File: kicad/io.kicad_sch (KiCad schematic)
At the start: 9 parts, among them SW1 UP, SW2 DOWN, SW3 OK, SW4 CANCEL

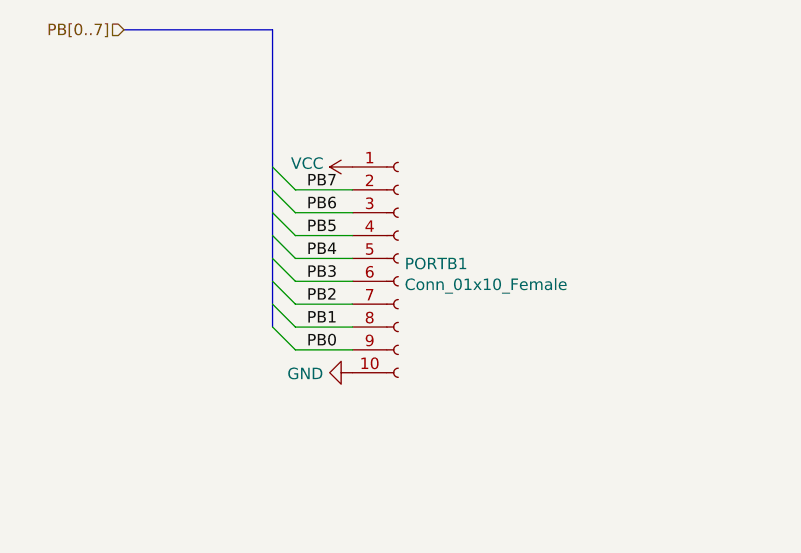
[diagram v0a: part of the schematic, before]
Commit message: Uploaded firmware v2.0.2
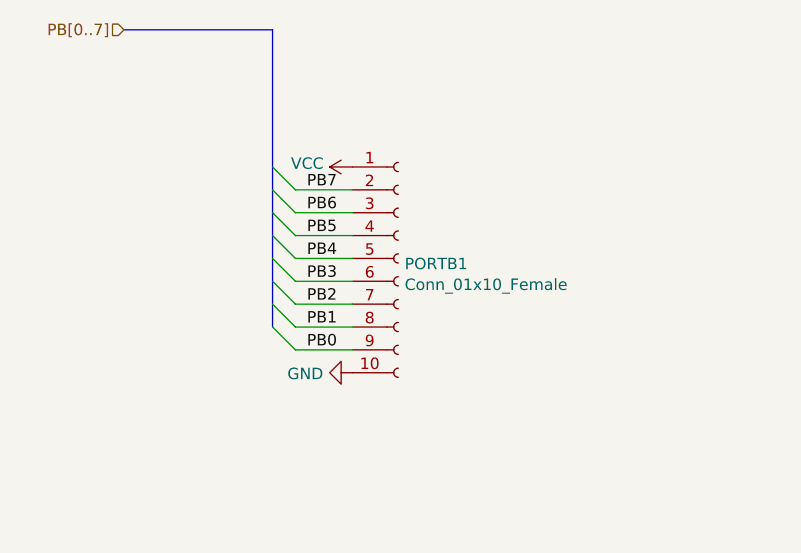
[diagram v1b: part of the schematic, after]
